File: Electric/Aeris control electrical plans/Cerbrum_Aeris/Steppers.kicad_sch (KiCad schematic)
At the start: 18 parts, among them J10 Conn_01x08_Stepper, J11 Conn_09x16_Stepper, J12 Conn_09x16_Stepper, J13 Conn_09x16_Stepper, J2 Conn_01x08_Stepper, J3 Conn_01x08_Stepper, J4 Conn_01x08_Stepper, J5 Conn_09x16_Stepper, J6 Conn_09x16_Stepper, J7 Conn_09x16_Stepper, J8 Conn_01x08_Stepper, J9 Conn_01x08_Stepper, M1 Stepper_Motor_bipolar, M2 Stepper_Motor_bipolar, M3 Stepper_Motor_bipolar, M4 Stepper_Motor_bipolar, M5 Stepper_Motor_bipolar, M6 Stepper_Motor_bipolar

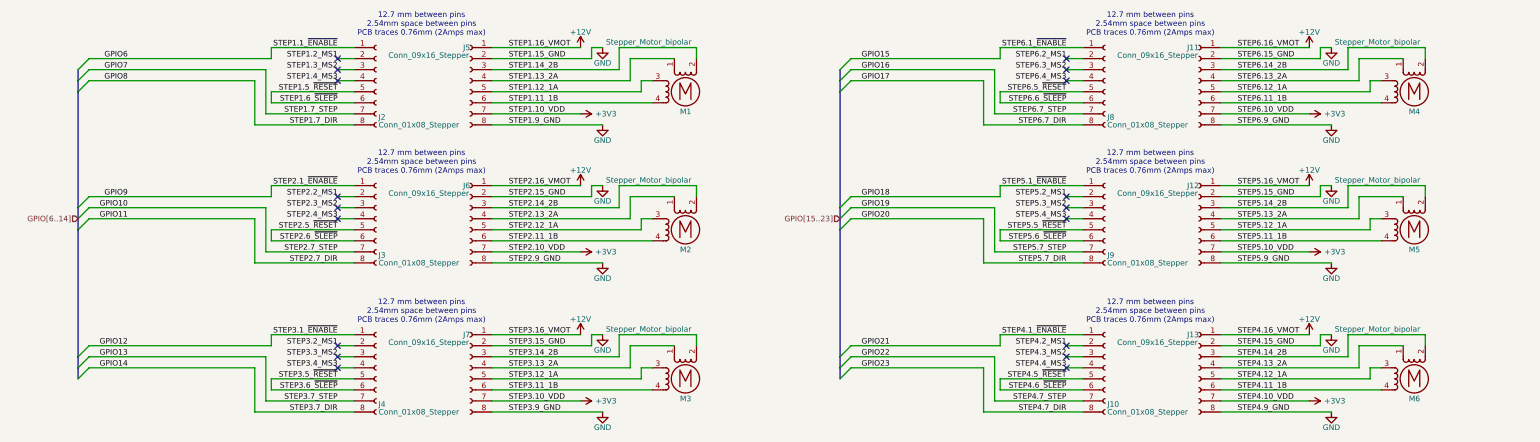
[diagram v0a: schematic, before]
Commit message: push éelectrique pcb
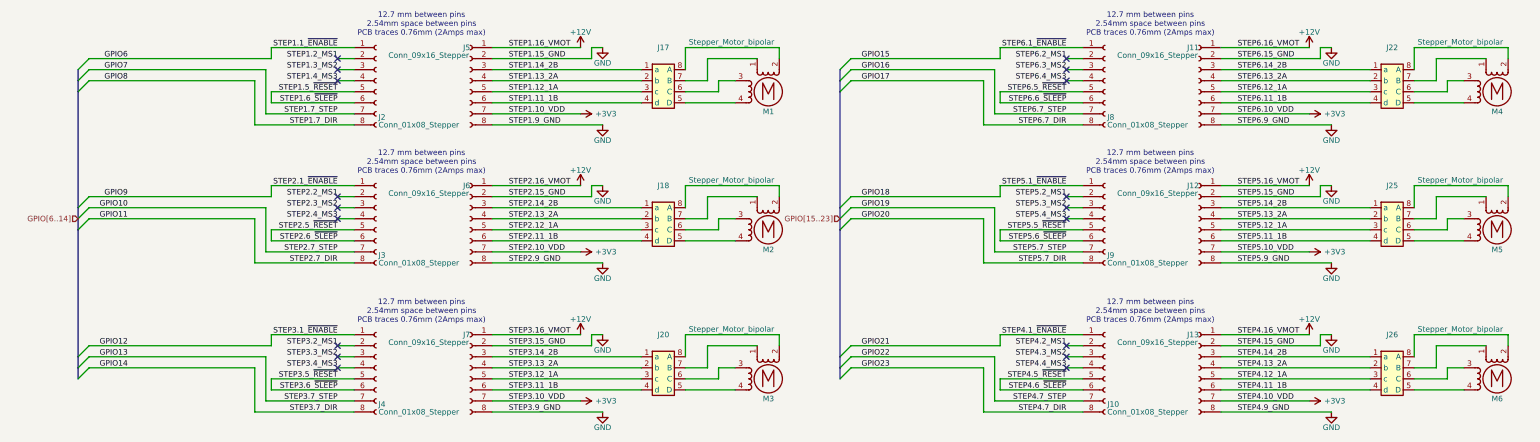
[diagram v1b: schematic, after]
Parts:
- added J17, J18, J20, J22, J25, J26: ~, Custom_Aeris:SJ_Stepper_1-5mm, symbol Aeris_custom:SJ_Stepper_1-5mm
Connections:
- net STEP1.11_1B: now also J17.4 (d); no longer M1.4
- net STEP1.12_1A: now also J17.3 (c); no longer M1.3
- net STEP1.13_2A: now also J17.2 (b); no longer M1.1
- net STEP1.14_2B: now also J17.1 (a); no longer M1.2 (-)
- net STEP2.11_1B: now also J18.4 (d); no longer M2.4
- net STEP2.12_1A: now also J18.3 (c); no longer M2.3
- net STEP2.13_2A: now also J18.2 (b); no longer M2.1
- net STEP2.14_2B: now also J18.1 (a); no longer M2.2 (-)
- net STEP3.11_1B: now also J20.4 (d); no longer M3.4
- net STEP3.12_1A: now also J20.3 (c); no longer M3.3
- net STEP3.13_2A: now also J20.2 (b); no longer M3.1
- net STEP3.14_2B: now also J20.1 (a); no longer M3.2 (-)
- net STEP4.11_1B: now also J26.4 (d); no longer M6.4
- net STEP4.12_1A: now also J26.3 (c); no longer M6.3
- net STEP4.13_2A: now also J26.2 (b); no longer M6.1
- net STEP4.14_2B: now also J26.1 (a); no longer M6.2 (-)
- net STEP5.11_1B: now also J25.4 (d); no longer M5.4
- net STEP5.12_1A: now also J25.3 (c); no longer M5.3
- net STEP5.13_2A: now also J25.2 (b); no longer M5.1
- net STEP5.14_2B: now also J25.1 (a); no longer M5.2 (-)
- net STEP6.11_1B: now also J22.4 (d); no longer M4.4
- net STEP6.12_1A: now also J22.3 (c); no longer M4.3
- net STEP6.13_2A: now also J22.2 (b); no longer M4.1
- net STEP6.14_2B: now also J22.1 (a); no longer M4.2 (-)
- new net: J17.5 (D), M1.4
- new net: J17.6 (C), M1.3
- new net: J17.7 (B), M1.1
- new net: J17.8 (A), M1.2 (-)
- new net: J20.7 (B), M3.1
- new net: J20.8 (A), M3.2 (-)
- new net: J20.6 (C), M3.3
- new net: J20.5 (D), M3.4
- new net: J22.7 (B), M4.1
- new net: J22.8 (A), M4.2 (-)
- new net: J22.6 (C), M4.3
- new net: J22.5 (D), M4.4
- new net: J18.7 (B), M2.1
- new net: J18.8 (A), M2.2 (-)
- new net: J18.6 (C), M2.3
- new net: J18.5 (D), M2.4
- new net: J25.5 (D), M5.4
- new net: J25.6 (C), M5.3
- new net: J25.7 (B), M5.1
- new net: J25.8 (A), M5.2 (-)
- new net: J26.7 (B), M6.1
- new net: J26.8 (A), M6.2 (-)
- new net: J26.6 (C), M6.3
- new net: J26.5 (D), M6.4
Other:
- moved on the sheet: M1
